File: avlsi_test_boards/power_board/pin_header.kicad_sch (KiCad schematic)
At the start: 3 parts, among them J5 Conn_01x02_Pin, J6 Conn_01x02_Pin

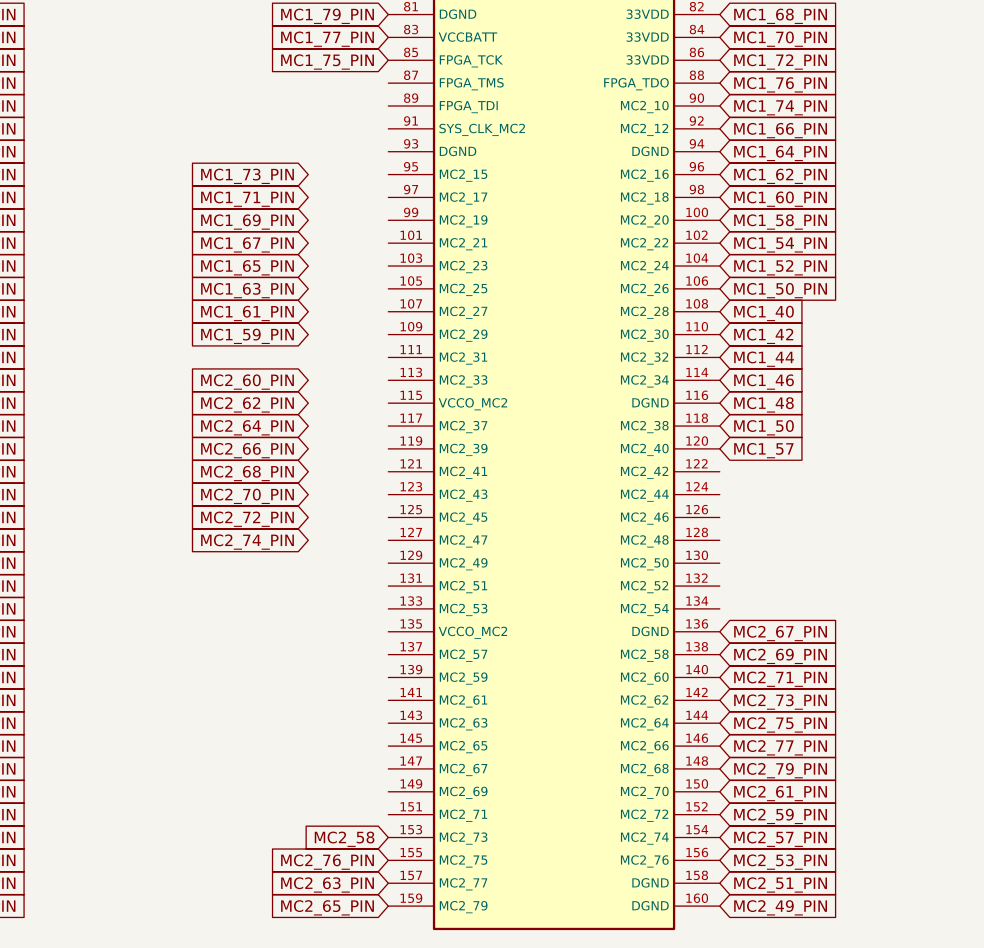
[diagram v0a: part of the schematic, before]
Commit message: Add updated pcb for second revision
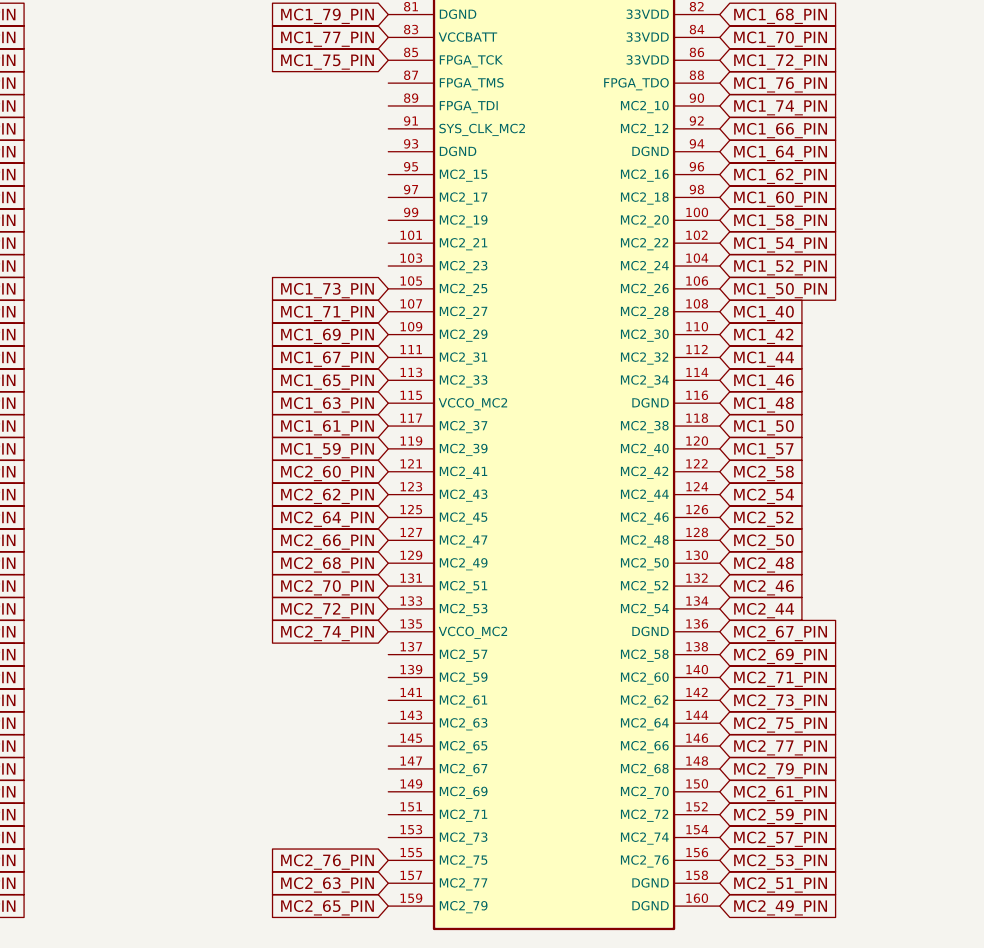
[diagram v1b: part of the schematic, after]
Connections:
- net MC1_59_PIN: now also U12.119 (MC2_39)
- net MC1_61_PIN: now also U12.117 (MC2_37)
- net MC1_63_PIN: now also U12.115 (VCCO_MC2)
- net MC1_65_PIN: now also U12.113 (MC2_33)
- net MC1_67_PIN: now also U12.111 (MC2_31)
- net MC1_69_PIN: now also U12.109 (MC2_29)
- net MC1_71_PIN: now also U12.107 (MC2_27)
- net MC1_73_PIN: now also U12.105 (MC2_25)
- net MC2_58: now also U12.122 (MC2_42); no longer U12.153 (MC2_73)
- net MC2_60_PIN: now also U12.121 (MC2_41)
- net MC2_62_PIN: now also U12.123 (MC2_43)
- net MC2_64_PIN: now also U12.125 (MC2_45)
- net MC2_66_PIN: now also U12.127 (MC2_47)
- net MC2_68_PIN: now also U12.129 (MC2_49)
- net MC2_70_PIN: now also U12.131 (MC2_51)
- net MC2_72_PIN: now also U12.133 (MC2_53)
- net MC2_74_PIN: now also U12.135 (VCCO_MC2)
- net MC2_54: now reaches U12.124 (MC2_44)
- net MC2_52: now reaches U12.126 (MC2_46)
- net MC2_50: now reaches U12.128 (MC2_48)
- net MC2_48: now reaches U12.130 (MC2_50)
- net MC2_46: now reaches U12.132 (MC2_52)
- net MC2_44: now reaches U12.134 (MC2_54)
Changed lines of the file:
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@@
 	(global_label "MC2_66_PIN"
 		(shape input)
-		(at 124.46 99.06 180)
+		(at 133.35 109.22 180)
 		(fields_autoplaced yes)
 		(effects
@@
 		)
 		(property "Intersheetrefs" "${INTERSHEET_REFS}"
-			(at 109.9844 99.06 0)
+			(at 118.8744 109.22 0)
 			(effects
 				(font
@@
 	(global_label "MC1_67_PIN"
 		(shape input)
-		(at 124.46 76.2 180)
+		(at 133.35 88.9 180)
 		(fields_autoplaced yes)
 		(effects
@@
 		)
 		(property "Intersheetrefs" "${INTERSHEET_REFS}"
-			(at 109.9844 76.2 0)
+			(at 118.8744 88.9 0)
 			(effects
 				(font
@@
 		)
 	)
+	(global_label "MC2_44"
+		(shape input)
+		(at 170.18 116.84 0)
+		(fields_autoplaced yes)
+		(effects
+			(font
+				(size 1.27 1.27)
+			)
+			(justify left)
+		)
+		(property "Intersheetrefs" "${INTERSHEET_REFS}"
+			(at 180.4827 116.84 0)
+			(effects
+				(font
+					(size 1.27 1.27)
+				)
+				(justify left)
+				(hide yes)
+			)
+		)
+	)
 	(global_label "FPGA_33VDD"
 		(shape input)
@@
 	(global_label "MC1_71_PIN"
 		(shape input)
-		(at 124.46 71.12 180)
+		(at 133.35 83.82 180)
 		(fields_autoplaced yes)
 		(effects
@@
 		)
 		(property "Intersheetrefs" "${INTERSHEET_REFS}"
-			(at 109.9844 71.12 0)
+			(at 118.8744 83.82 0)
 			(effects
 				(font
@@
 	(global_label "MC1_69_PIN"
 		(shape input)
-		(at 124.46 73.66 180)
+		(at 133.35 86.36 180)
 		(fields_autoplaced yes)
 		(effects
@@
 		)
 		(property "Intersheetrefs" "${INTERSHEET_REFS}"
-			(at 109.9844 73.66 0)
+			(at 118.8744 86.36 0)
 			(effects
 				(font
@@
 	(global_label "MC2_64_PIN"
 		(shape input)
-		(at 124.46 96.52 180)
+		(at 133.35 106.68 180)
 		(fields_autoplaced yes)
 		(effects
@@
 		)
 		(property "Intersheetrefs" "${INTERSHEET_REFS}"
-			(at 109.9844 96.52 0)
+			(at 118.8744 106.68 0)
 			(effects
 				(font
@@
 	(global_label "MC1_59_PIN"
 		(shape input)
-		(at 124.46 86.36 180)
+		(at 133.35 99.06 180)
 		(fields_autoplaced yes)
 		(effects
@@
 		)
 		(property "Intersheetrefs" "${INTERSHEET_REFS}"
-			(at 109.9844 86.36 0)
+			(at 118.8744 99.06 0)
 			(effects
 				(font
@@
 	(global_label "MC2_68_PIN"
 		(shape input)
-		(at 124.46 101.6 180)
+		(at 133.35 111.76 180)
 		(fields_autoplaced yes)
 		(effects
@@
 		)
 		(property "Intersheetrefs" "${INTERSHEET_REFS}"
-			(at 109.9844 101.6 0)
+			(at 118.8744 111.76 0)
 			(effects
 				(font
@@
 		)
 	)
+	(global_label "MC2_54"
+		(shape input)
+		(at 170.18 104.14 0)
+		(fields_autoplaced yes)
+		(effects
+			(font
+				(size 1.27 1.27)
+			)
+			(justify left)
+		)
+		(property "Intersheetrefs" "${INTERSHEET_REFS}"
+			(at 180.4827 104.14 0)
+			(effects
+				(font
+					(size 1.27 1.27)
+				)
+				(justify left)
+				(hide yes)
+			)
+		)
+	)
 	(global_label "VCCA09"
 		(shape input)
@@
 		)
 	)
-	(global_label "MC2_58"
-		(shape input)
-		(at 133.35 142.24 180)
-		(fields_autoplaced yes)
-		(effects
-			(font
-				(size 1.27 1.27)
-			)
-			(justify right)
-		)
-		(property "Intersheetrefs" "${INTERSHEET_REFS}"
-			(at 123.0473 142.24 0)
-			(effects
-				(font
-					(size 1.27 1.27)
-				)
-				(justify right)
-				(hide yes)
-			)
-		)
-	)
 	(global_label "MC1_40"
 		(shape input)
@@
 	(global_label "MC1_73_PIN"
 		(shape input)
-		(at 124.46 68.58 180)
+		(at 133.35 81.28 180)
 		(fields_autoplaced yes)
 		(effects
@@
 		)
 		(property "Intersheetrefs" "${INTERSHEET_REFS}"
-			(at 109.9844 68.58 0)
+			(at 118.8744 81.28 0)
 			(effects
 				(font
@@
 	(global_label "MC2_60_PIN"
 		(shape input)
-		(at 124.46 91.44 180)
+		(at 133.35 101.6 180)
 		(fields_autoplaced yes)
 		(effects
@@
 		)
 		(property "Intersheetrefs" "${INTERSHEET_REFS}"
-			(at 109.9844 91.44 0)
+			(at 118.8744 101.6 0)
 			(effects
 				(font
@@
 	(global_label "MC2_70_PIN"
 		(shape input)
-		(at 124.46 104.14 180)
+		(at 133.35 114.3 180)
 		(fields_autoplaced yes)
 		(effects
@@
 		)
 		(property "Intersheetrefs" "${INTERSHEET_REFS}"
-			(at 109.9844 104.14 0)
+			(at 118.8744 114.3 0)
 			(effects
 				(font
@@
 	(global_label "MC2_72_PIN"
 		(shape input)
-		(at 124.46 106.68 180)
+		(at 133.35 116.84 180)
 		(fields_autoplaced yes)
 		(effects
@@
 		)
 		(property "Intersheetrefs" "${INTERSHEET_REFS}"
-			(at 109.9844 106.68 0)
+			(at 118.8744 116.84 0)
 			(effects
 				(font
@@
 		)
 	)
+	(global_label "MC2_52"
+		(shape input)
+		(at 170.18 106.68 0)
+		(fields_autoplaced yes)
+		(effects
+			(font
+				(size 1.27 1.27)
+			)
+			(justify left)
+		)
+		(property "Intersheetrefs" "${INTERSHEET_REFS}"
+			(at 180.4827 106.68 0)
+			(effects
+				(font
+					(size 1.27 1.27)
+				)
+				(justify left)
+				(hide yes)
+			)
+		)
+	)
 	(global_label "MC1_33_PIN"
 		(shape input)
@@
 	(global_label "MC1_65_PIN"
 		(shape input)
-		(at 124.46 78.74 180)
+		(at 133.35 91.44 180)
 		(fields_autoplaced yes)
 		(effects
@@
 		)
 		(property "Intersheetrefs" "${INTERSHEET_REFS}"
-			(at 109.9844 78.74 0)
+			(at 118.8744 91.44 0)
 			(effects
 				(font
@@
 		)
 	)
+	(global_label "MC2_50"
+		(shape input)
+		(at 170.18 109.22 0)
+		(fields_autoplaced yes)
+		(effects
+			(font
+				(size 1.27 1.27)
+			)
+			(justify left)
+		)
+		(property "Intersheetrefs" "${INTERSHEET_REFS}"
+			(at 180.4827 109.22 0)
+			(effects
+				(font
+					(size 1.27 1.27)
+				)
+				(justify left)
+				(hide yes)
+			)
+		)
+	)
 	(global_label "MC1_46"
 		(shape input)
@@
 	(global_label "MC1_61_PIN"
 		(shape input)
-		(at 124.46 83.82 180)
+		(at 133.35 96.52 180)
 		(fields_autoplaced yes)
 		(effects
@@
 		)
 		(property "Intersheetrefs" "${INTERSHEET_REFS}"
-			(at 109.9844 83.82 0)
+			(at 118.8744 96.52 0)
 			(effects
 				(font
@@
 	(global_label "MC2_74_PIN"
 		(shape input)
-		(at 124.46 109.22 180)
+		(at 133.35 119.38 180)
 		(fields_autoplaced yes)
 		(effects
@@
 		)
 		(property "Intersheetrefs" "${INTERSHEET_REFS}"
-			(at 109.9844 109.22 0)
+			(at 118.8744 119.38 0)
 			(effects
 				(font
@@
 		)
 	)
+	(global_label "MC2_58"
+		(shape input)
+		(at 170.18 101.6 0)
+		(fields_autoplaced yes)
+		(effects
+			(font
+				(size 1.27 1.27)
+			)
+			(justify left)
+		)
+		(property "Intersheetrefs" "${INTERSHEET_REFS}"
+			(at 180.4827 101.6 0)
+			(effects
+				(font
+					(size 1.27 1.27)
+				)
+				(justify left)
+				(hide yes)
+			)
+		)
+	)
+	(global_label "MC2_46"
+		(shape input)
+		(at 170.18 114.3 0)
+		(fields_autoplaced yes)
+		(effects
+			(font
+				(size 1.27 1.27)
+			)
+			(justify left)
+		)
+		(property "Intersheetrefs" "${INTERSHEET_REFS}"
+			(at 180.4827 114.3 0)
+			(effects
+				(font
+					(size 1.27 1.27)
+				)
+				(justify left)
+				(hide yes)
+			)
+		)
+	)
 	(global_label "MC2_10_PIN"
 		(shape input)
@@
 		)
 	)
+	(global_label "MC2_48"
+		(shape input)
+		(at 170.18 111.76 0)
+		(fields_autoplaced yes)
+		(effects
+			(font
+				(size 1.27 1.27)
+			)
+			(justify left)
+		)
+		(property "Intersheetrefs" "${INTERSHEET_REFS}"
+			(at 180.4827 111.76 0)
+			(effects
+				(font
+					(size 1.27 1.27)
+				)
+				(justify left)
+				(hide yes)
+			)
+		)
+	)
 	(global_label "FPGA_TCK"
 		(shape input)
@@
 	(global_label "MC1_63_PIN"
 		(shape input)
-		(at 124.46 81.28 180)
+		(at 133.35 93.98 180)
 		(fields_autoplaced yes)
 		(effects
@@
 		)
 		(property "Intersheetrefs" "${INTERSHEET_REFS}"
-			(at 109.9844 81.28 0)
+			(at 118.8744 93.98 0)
 			(effects
 				(font
@@
 	(global_label "MC2_62_PIN"
 		(shape input)
-		(at 124.46 93.98 180)
+		(at 133.35 104.14 180)
 		(fields_autoplaced yes)
 		(effects
@@
 		)
 		(property "Intersheetrefs" "${INTERSHEET_REFS}"
-			(at 109.9844 93.98 0)
+			(at 118.8744 104.14 0)
 			(effects
 				(font
